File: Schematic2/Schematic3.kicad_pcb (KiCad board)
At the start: 2 copper layers, 100 x 119 mm, 52 parts, among them SW1 Rotary_Encoder_Switch, U1 Kailhlowprofile, U10 Kailhlowprofile, U11 Kailhlowprofile, U12 Kailhlowprofile, U13 Kailhlowprofile, U14 Kailhlowprofile, U15 Kailhlowprofile, U16 Kailhlowprofile, U17 Kailhlowprofile, U18 Kailhlowprofile, U19 Kailhlowprofile, U2 Kailhlowprofile, U20 Kailhlowprofile, U3 Kailhlowprofile, U4 Kailhlowprofile, U5 Kailhlowprofile, U6 Kailhlowprofile, U7 Kailhlowprofile, U8 Kailhlowprofile, U9 Kailhlowprofile

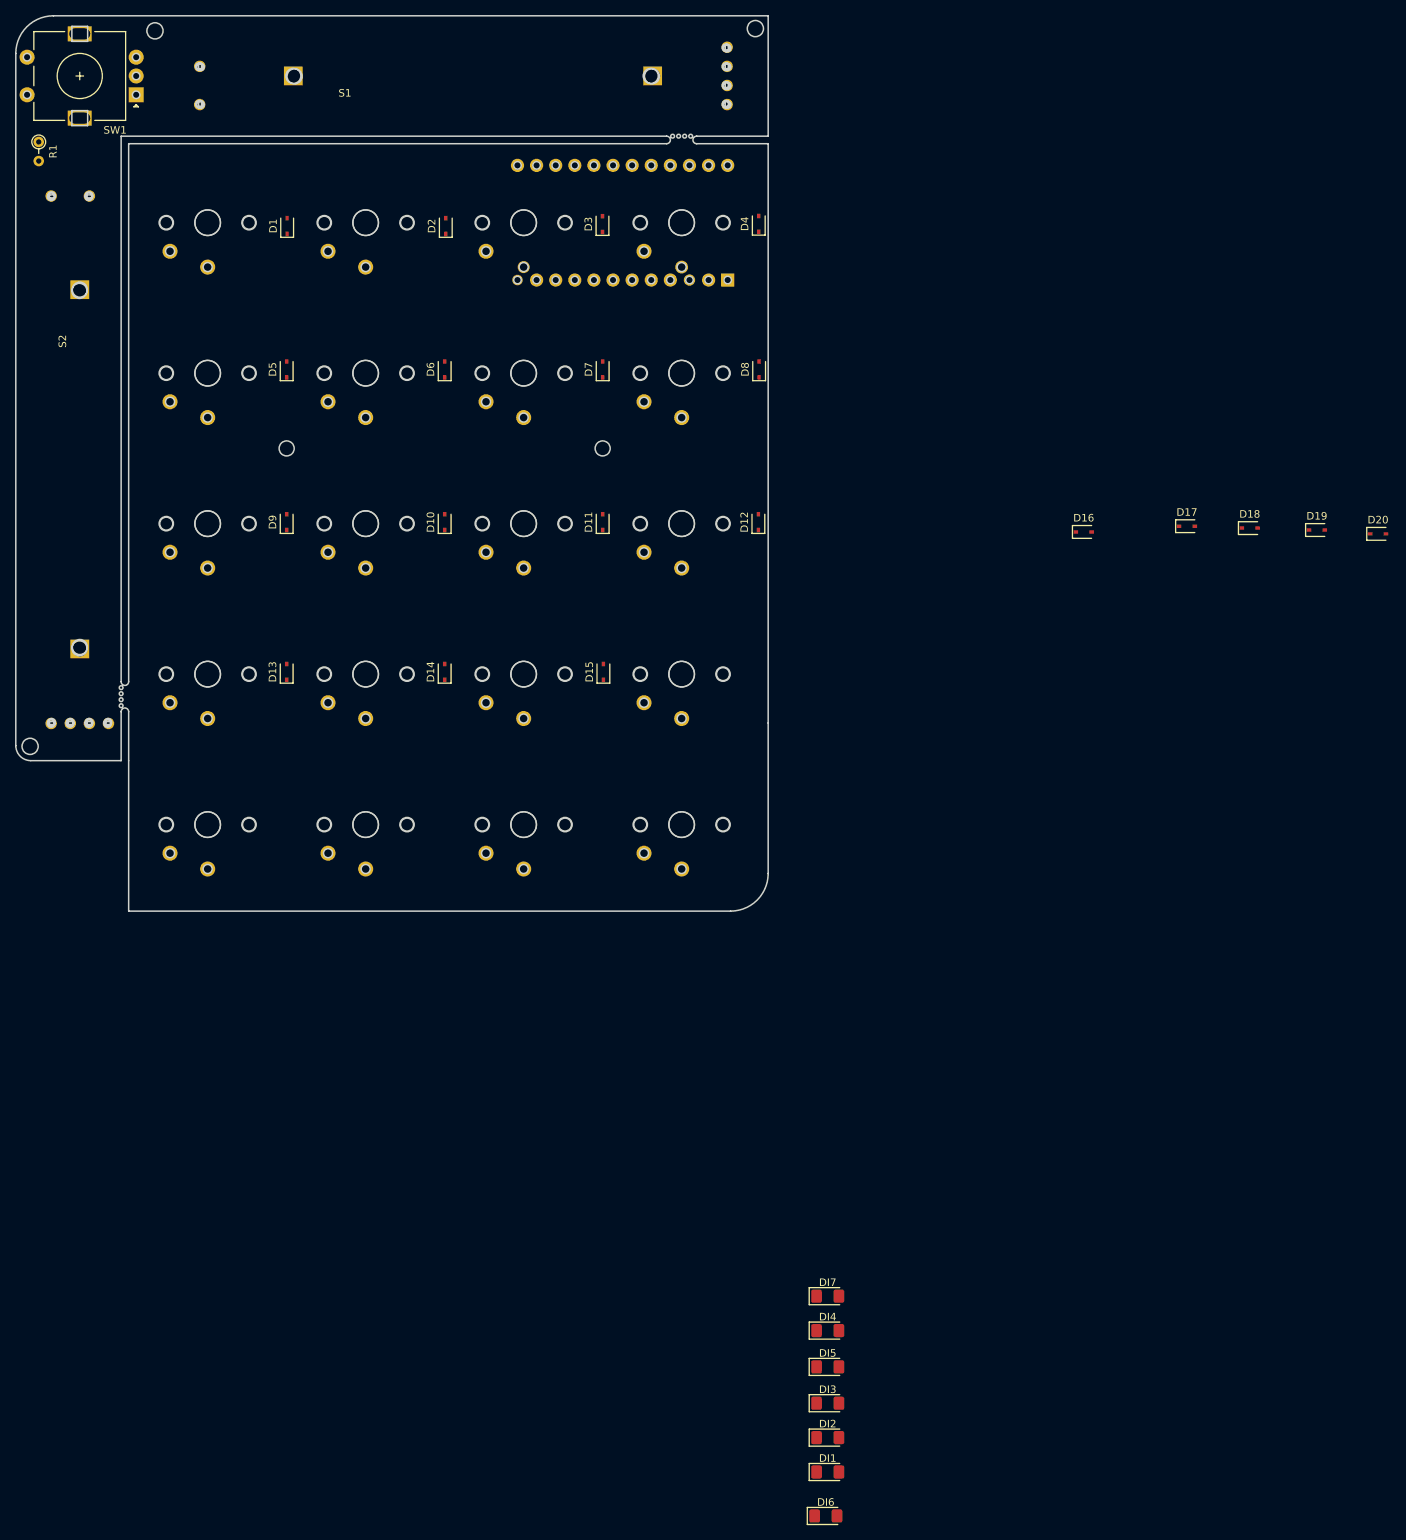
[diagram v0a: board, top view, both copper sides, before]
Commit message: The final countdown
The diamond deluxe of FINAL
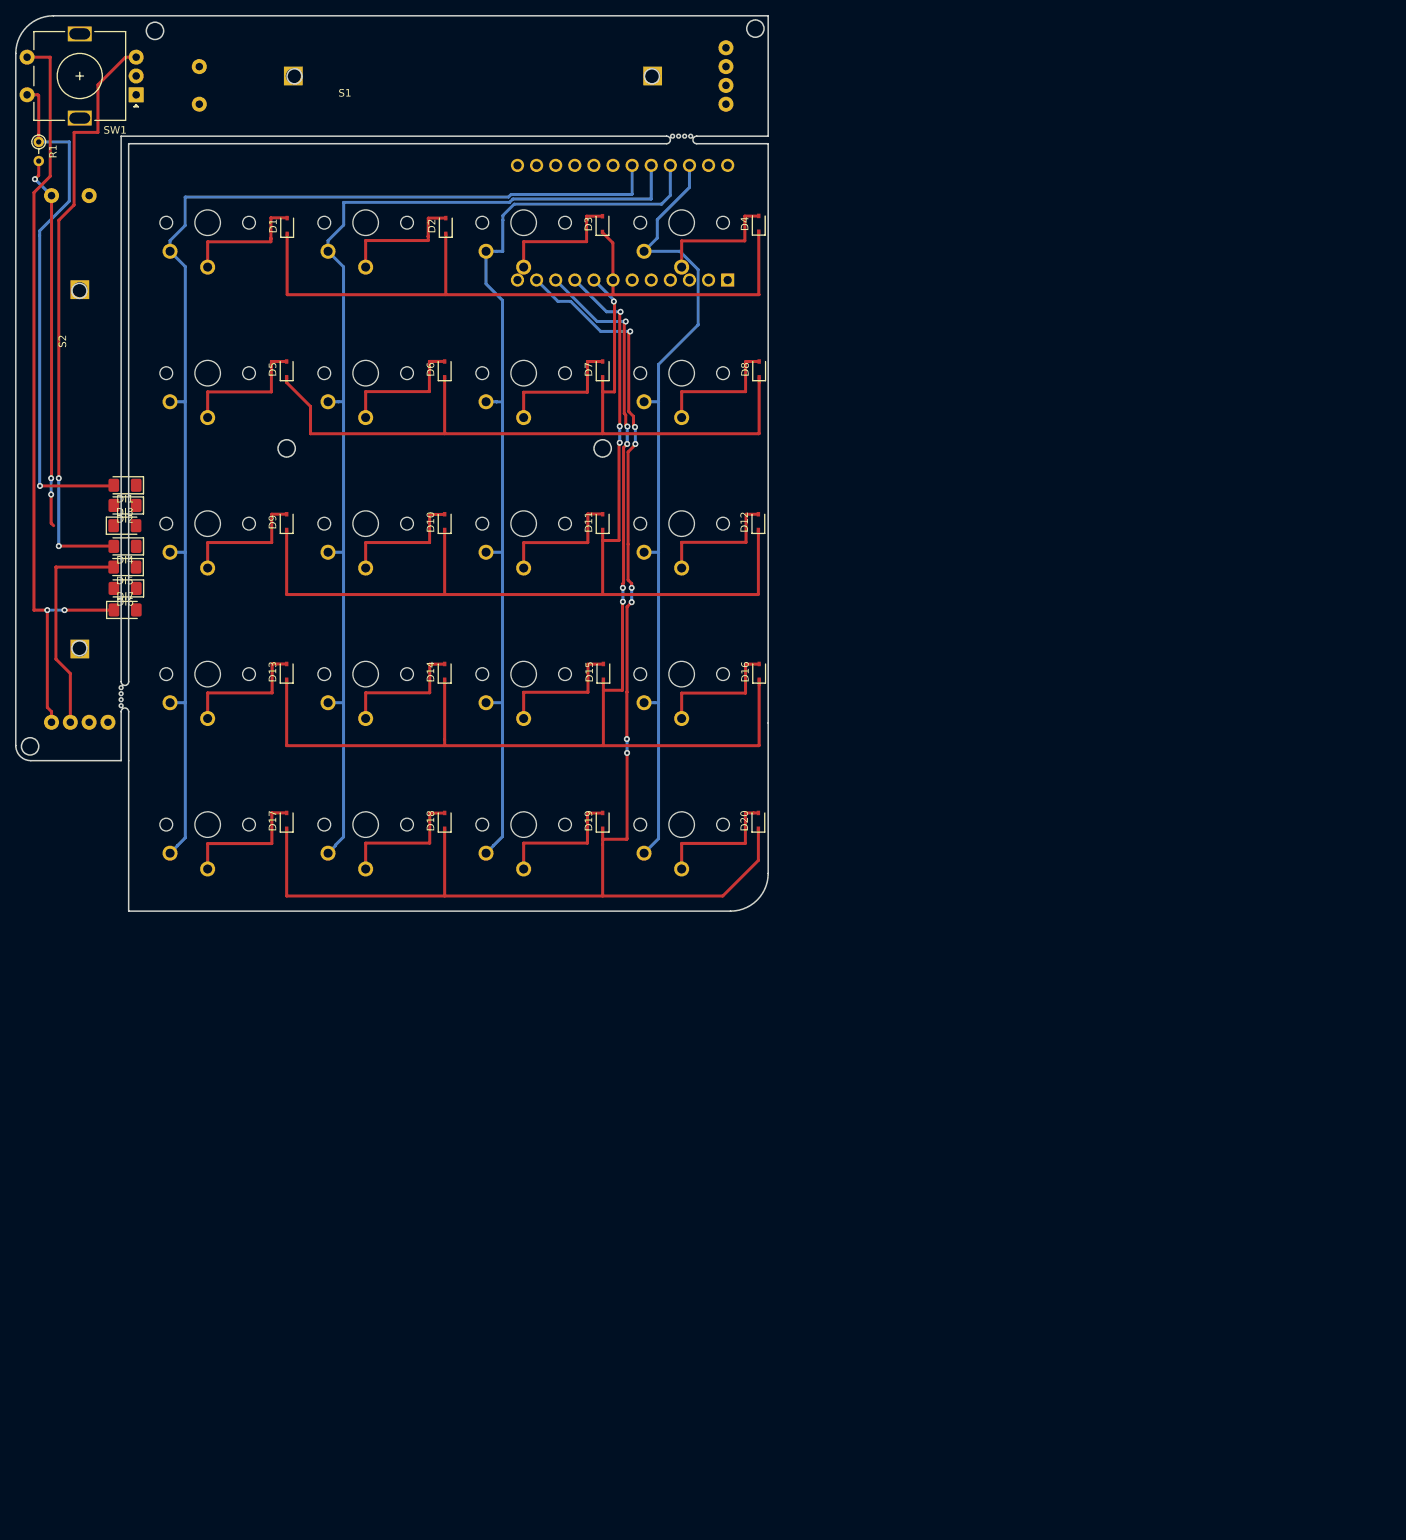
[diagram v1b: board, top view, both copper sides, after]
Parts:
- moved DI1 161.0 mm to (14.5, 62.4), turned to 180 degrees
- moved DI2 155.2 mm to (14.5, 65.1), turned to 180 degrees
- moved DI6 154.5 mm to (14.5, 76.1), turned to 180 degrees
- moved DI3 149.4 mm to (14.5, 67.8)
- moved DI5 141.5 mm to (14.5, 73.3), turned to 180 degrees
- moved DI4 140.0 mm to (14.5, 70.5), turned to 180 degrees
- moved DI7 130.5 mm to (14.5, 79.0)
- moved D17 125.9 mm to (36.0, 107.0), turned to 90 degrees
- moved D18 113.9 mm to (57.0, 107.0), turned to 90 degrees
- moved D19 102.5 mm to (78.0, 107.0), turned to 90 degrees
- moved D20 90.8 mm to (98.7, 107.0), turned to 90 degrees
- moved D16 47.0 mm to (98.8, 87.2), turned to 90 degrees
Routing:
- net R5: track 0.00 -> 183.0 mm, vias 0 -> 7
- net R4: track 0.00 -> 161.5 mm, vias 0 -> 5
- net C1: track 0.00 -> 159.2 mm
- net C2: track 0.11 -> 140.9 mm
- net R3: track 0.00 -> 137.4 mm, vias 0 -> 3
- net C3: track 0.00 -> 122.8 mm
- net R2: track 0.00 -> 108.5 mm, vias 0 -> 1
- net C4: track 0.00 -> 108.5 mm
- net S1: track 0.00 -> 103.2 mm, vias 0 -> 2
- net R1: track 0.00 -> 96.2 mm
- net Net-(DI4-Pad2): track 0.00 -> 79.3 mm, vias 0 -> 2
- net Net-(DI1-Pad2): track 0.00 -> 69.0 mm, vias 0 -> 1
- net EnGNDC1: track 0.00 -> 49.8 mm, vias 0 -> 3
- net Net-(DI5-Pad2): track 0.00 -> 29.1 mm
- net Net-(D17-Pad2): track 0.00 -> 18.0 mm
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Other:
- outline, holes or cut-outs redrawn
